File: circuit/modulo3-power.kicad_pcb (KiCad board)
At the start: 2 copper layers, 0 parts

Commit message: fv-1 mostly done; power progressed
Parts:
- added BT1: 25V, myAmp:XT60-M, F.Cu at (107.3, 97.2)
- added C1: 100nF, myAmp:C_1206, F.Cu at (62.9, 67.3)
- added C10: 47μF, myAmp:CPOL_D4_P1.5, F.Cu at (96.5, 59.1)
- added C2: 330n, myAmp:C_5.0MM, F.Cu at (120.7, 85.7)
- added C3: 100nF, myAmp:C_1206, F.Cu at (61.6, 80.0)
- added C4: 20μF, myAmp:CPOL_D6.3_P2.5, F.Cu at (57.1, 80.0)
- added C5: 20μF, myAmp:CPOL_D6.3_P2.5, F.Cu at (66.0, 80.0)
- added C6: 10μF, myAmp:C_1812, F.Cu at (68.6, 64.1)
- added C7: 10μF, myAmp:C_1812, F.Cu at (72.4, 64.1)
- added C8: 100nF, myAmp:C_1206, F.Cu at (96.5, 62.9)
- added C9: 10μF, myAmp:CPOL_D4_P1.5, F.Cu at (101.6, 65.4)
- added D1: 1N4148, myAmp:DO35, F.Cu at (65.4, 64.1)
- added D2: SS18A, myAmp:D_SMA, F.Cu at (57.8, 72.4)
- added D3: power, myAmp:LED_D3.0mm, F.Cu at (92.1, 97.8)
- added F1: 2A, myAmp:MF-LSMF, F.Cu at (106.7, 87.0)
- added J1: HOLE, myAmp:MountingHole, F.Cu at (54.0, 54.0)
- added J2: HOLE, myAmp:MountingHole, F.Cu at (130.0, 54.0)
- added J3: HOLE, myAmp:MountingHole, F.Cu at (54.0, 98.0)
- added J4: HOLE, myAmp:MountingHole, F.Cu at (130.0, 98.0)
- added L1: 27μH, myAmp:COIL_DER0705, F.Cu at (69.2, 72.4)
- added Q1: IRF4905SPBF, myAmp:D2PAK, F.Cu at (120.7, 73.7)
- added R1: 470k, myAmp:R_10MM, F.Cu at (120.7, 88.9)
- added R2: 75K, myAmp:R_0805, F.Cu at (61.0, 62.2)
- added R3: 10K, myAmp:R_0805, F.Cu at (58.4, 62.2)
- added R4: 1M, myAmp:R_10MM, F.Cu at (120.7, 91.4)
- added R5: 4k7, myAmp:R_10MM, F.Cu at (82.5, 97.8)
- added SW1: on/off, myAmp:SW_DPDT, F.Cu at (120.7, 98.0)
- added U1: MCP16331, myAmp:SOT-23-6, F.Cu at (59.7, 67.3)
- added U2: LM1117-5.0, myAmp:TO-252-3, F.Cu at (107.4, 59.7)
- added U3: PWR_CONN, myAmp:PWR_CONN, F.Cu at (121.0, 54.0)
- added U4: AMPCTRL, myAmp:AMPCTRL, F.Cu at (76.0, 54.0)
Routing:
- added copper zone on B.Cu, net GND
- added copper zone on F.Cu, net GND
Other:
- board outline added: 84 x 52 mm

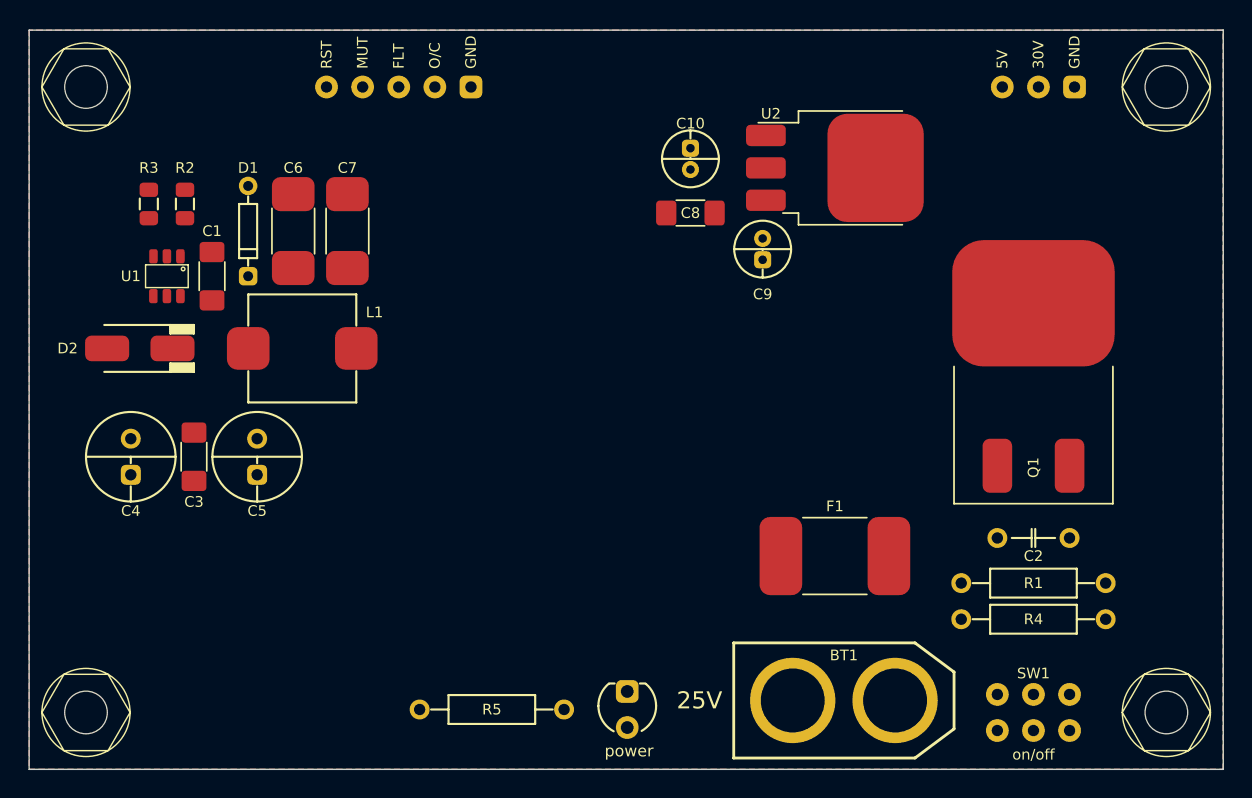
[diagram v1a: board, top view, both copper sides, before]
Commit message: lotsa things :)
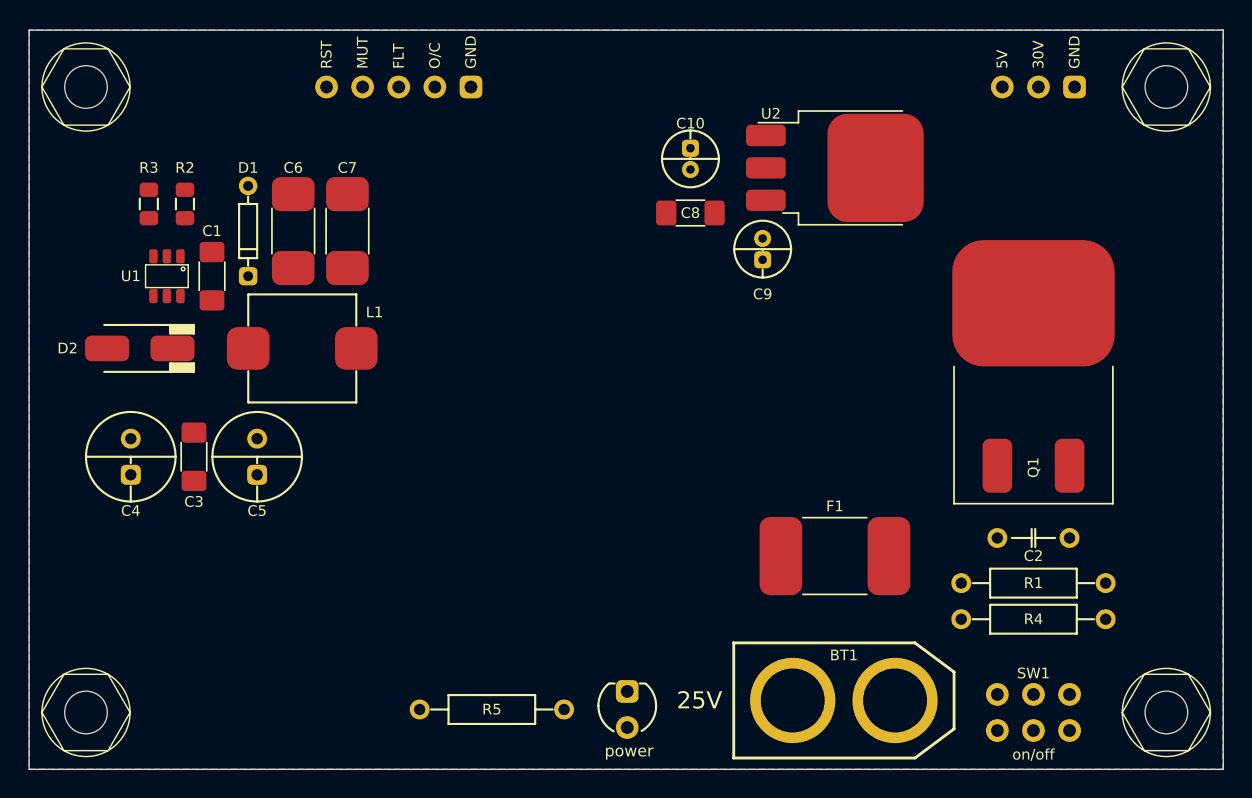
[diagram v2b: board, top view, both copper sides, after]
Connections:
- SW1 pad 5: unconnected-(SW1-Pad5) -> /MUTE
- SW1 pad 6: unconnected-(SW1-Pad6) -> GND
- U4 pad 3: unconnected-(U4-MUTE-Pad3) -> /MUTE
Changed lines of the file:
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@@
   (net 13 "unconnected-(U1-EN-Pad4)")
   (net 14 "unconnected-(U4-RESET-Pad2)")
-  (net 15 "unconnected-(U4-MUTE-Pad3)")
+  (net 15 "/MUTE")
   (net 16 "unconnected-(U4-FAULT-Pad4)")
   (net 17 "unconnected-(U4-OTW_CLIP-Pad5)")
   (net 18 "unconnected-(SW1-Pad3)")
   (net 19 "unconnected-(SW1-Pad4)")
-  (net 20 "unconnected-(SW1-Pad5)")
-  (net 21 "unconnected-(SW1-Pad6)")
   (footprint "myAmp:C_1812" (layer "F.Cu")
     (at 68.58 64.135 90)
@@
         (effects (font (size 0.75 0.75) (thickness 0.15)))
     )
-    (pad "1" thru_hole circle (at -1.27 2.54) (size 1.6 1.6) (drill 0.8) (layers "*.Cu" "*.Mask")
+    (pad "1" thru_hole circle (at -1.27 2.54) (size 1.6 1.6) (drill 0.9) (layers "*.Cu" "*.Mask")
       (net 5 "Net-(Q1-S)") (pintype "passive"))
-    (pad "2" thru_hole circle (at -1.27 0) (size 1.6 1.6) (drill 0.8) (layers "*.Cu" "*.Mask")
+    (pad "2" thru_hole circle (at -1.27 0) (size 1.6 1.6) (drill 0.9) (layers "*.Cu" "*.Mask")
       (net 11 "Net-(F1-Pad2)") (pintype "passive"))
-    (pad "3" thru_hole circle (at -1.27 -2.54) (size 1.6 1.6) (drill 0.8) (layers "*.Cu" "*.Mask")
+    (pad "3" thru_hole circle (at -1.27 -2.54) (size 1.6 1.6) (drill 0.9) (layers "*.Cu" "*.Mask")
       (net 18 "unconnected-(SW1-Pad3)") (pintype "passive+no_connect"))
-    (pad "4" thru_hole circle (at 1.27 2.54) (size 1.6 1.6) (drill 0.8) (layers "*.Cu" "*.Mask")
+    (pad "4" thru_hole circle (at 1.27 2.54) (size 1.6 1.6) (drill 0.9) (layers "*.Cu" "*.Mask")
       (net 19 "unconnected-(SW1-Pad4)") (pintype "passive+no_connect"))
-    (pad "5" thru_hole circle (at 1.27 0) (size 1.6 1.6) (drill 0.8) (layers "*.Cu" "*.Mask")
-      (net 20 "unconnected-(SW1-Pad5)") (pintype "passive"))
-    (pad "6" thru_hole circle (at 1.27 -2.54) (size 1.6 1.6) (drill 0.8) (layers "*.Cu" "*.Mask")
-      (net 21 "unconnected-(SW1-Pad6)") (pintype "passive"))
+    (pad "5" thru_hole circle (at 1.27 0) (size 1.6 1.6) (drill 0.9) (layers "*.Cu" "*.Mask")
+      (net 15 "/MUTE") (pintype "passive"))
+    (pad "6" thru_hole circle (at 1.27 -2.54) (size 1.6 1.6) (drill 0.9) (layers "*.Cu" "*.Mask")
+      (net 1 "GND") (pintype "passive"))
     (model "${KIPRJMOD}/myAmp.pretty/models/PinHeader_2x03_P2.54mm_Horizontal.wrl"
       (offset (xyz -1.27 2.54 0))
@@
     )
   )
-  (footprint "myAmp:AMPCTRL" (layer "F.Cu")
-    (at 76 54)
-    (property "Sheetfile" "modulo3-power.kicad_sch")
-    (property "Sheetname" "")
-    (attr through_hole)
-    (fp_text reference "U4" (at -7.62 0 unlocked) (layer "F.SilkS") hide
-        (effects (font (size 0.75 0.75) (thickness 0.15)))
-    )
-    (fp_text value "AMPCTRL" (at 0 1 unlocked) (layer "F.Fab") hide
-        (effects (font (size 1 1) (thickness 0.15)))
-    )
-    (fp_text user "FLT" (at 0 -1.27 90 unlocked) (layer "F.SilkS")
-        (effects (font (size 0.75 0.75) (thickness 0.15)) (justify left))
-    )
-    (fp_text user "MUT" (at -2.54 -1.27 90 unlocked) (layer "F.SilkS")
-        (effects (font (size 0.75 0.75) (thickness 0.15)) (justify left))
-    )
-    (fp_text user "GND" (at 5.08 -1.27 90 unlocked) (layer "F.SilkS")
-        (effects (font (size 0.75 0.75) (thickness 0.15)) (justify left))
-    )
-    (fp_text user "O/C" (at 2.54 -1.27 90 unlocked) (layer "F.SilkS")
-        (effects (font (size 0.75 0.75) (thickness 0.15)) (justify left))
-    )
-    (fp_text user "RST" (at -5.08 -1.27 90 unlocked) (layer "F.SilkS")
-        (effects (font (size 0.75 0.75) (thickness 0.15)) (justify left))
-    )
-    (pad "1" thru_hole roundrect (at 5.08 0) (size 1.6 1.6) (drill 0.8) (layers "*.Cu" "*.Mask") (roundrect_rratio 0.25)
-      (net 1 "GND") (pinfunction "GND") (pintype "input"))
-    (pad "2" thru_hole circle (at -5.08 0) (size 1.6 1.6) (drill 0.8) (layers "*.Cu" "*.Mask")
-      (net 14 "unconnected-(U4-RESET-Pad2)") (pinfunction "RESET") (pintype "input"))
-    (pad "3" thru_hole circle (at -2.54 0) (size 1.6 1.6) (drill 0.8) (layers "*.Cu" "*.Mask")
-      (net 15 "unconnected-(U4-MUTE-Pad3)") (pinfunction "MUTE") (pintype "input"))
-    (pad "4" thru_hole circle (at 0 0) (size 1.6 1.6) (drill 0.8) (layers "*.Cu" "*.Mask")
-      (net 16 "unconnected-(U4-FAULT-Pad4)") (pinfunction "FAULT") (pintype "output+no_connect"))
-    (pad "5" thru_hole circle (at 2.54 0) (size 1.6 1.6) (drill 0.8) (layers "*.Cu" "*.Mask")
-      (net 17 "unconnected-(U4-OTW_CLIP-Pad5)") (pinfunction "OTW_CLIP") (pintype "output+no_connect"))
-    (model "${KIPRJMOD}/myAmp.pretty/models/PinHeader_1x05_P2.54mm_Vertical.wrl"
-      (offset (xyz 5.08 0 0))
-      (scale (xyz 1 1 1))
-      (rotate (xyz 0 0 90))
-    )
-  )
   (footprint "myAmp:MountingHole" (layer "F.Cu")
     (at 54 54)
@@
       (scale (xyz 1 1 1))
       (rotate (xyz 0 0 0))
+    )
+  )
+  (footprint "myAmp:AMPCTRL" (layer "F.Cu")
+    (at 76 54)
+    (property "Sheetfile" "modulo3-power.kicad_sch")
+    (property "Sheetname" "")
+    (attr through_hole)
+    (fp_text reference "U4" (at -7.62 0 unlocked) (layer "F.SilkS") hide
+        (effects (font (size 0.75 0.75) (thickness 0.15)))
+    )
+    (fp_text value "AMPCTRL" (at 0 1 unlocked) (layer "F.Fab") hide
+        (effects (font (size 1 1) (thickness 0.15)))
+    )
+    (fp_text user "O/C" (at 2.54 -1.27 90 unlocked) (layer "F.SilkS")
+        (effects (font (size 0.75 0.75) (thickness 0.15)) (justify left))
+    )
+    (fp_text user "RST" (at -5.08 -1.27 90 unlocked) (layer "F.SilkS")
+        (effects (font (size 0.75 0.75) (thickness 0.15)) (justify left))
+    )
+    (fp_text user "FLT" (at 0 -1.27 90 unlocked) (layer "F.SilkS")
+        (effects (font (size 0.75 0.75) (thickness 0.15)) (justify left))
+    )
+    (fp_text user "GND" (at 5.08 -1.27 90 unlocked) (layer "F.SilkS")
+        (effects (font (size 0.75 0.75) (thickness 0.15)) (justify left))
+    )
+    (fp_text user "MUT" (at -2.54 -1.27 90 unlocked) (layer "F.SilkS")
+        (effects (font (size 0.75 0.75) (thickness 0.15)) (justify left))
+    )
+    (pad "1" thru_hole roundrect (at 5.08 0) (size 1.6 1.6) (drill 0.9) (layers "*.Cu" "*.Mask") (roundrect_rratio 0.25)
+      (net 1 "GND") (pinfunction "GND") (pintype "input"))
+    (pad "2" thru_hole circle (at -5.08 0) (size 1.6 1.6) (drill 0.9) (layers "*.Cu" "*.Mask")
+      (net 14 "unconnected-(U4-RESET-Pad2)") (pinfunction "RESET") (pintype "input+no_connect"))
+    (pad "3" thru_hole circle (at -2.54 0) (size 1.6 1.6) (drill 0.9) (layers "*.Cu" "*.Mask")
+      (net 15 "/MUTE") (pinfunction "MUTE") (pintype "input"))
+    (pad "4" thru_hole circle (at 0 0) (size 1.6 1.6) (drill 0.9) (layers "*.Cu" "*.Mask")
+      (net 16 "unconnected-(U4-FAULT-Pad4)") (pinfunction "FAULT") (pintype "output+no_connect"))
+    (pad "5" thru_hole circle (at 2.54 0) (size 1.6 1.6) (drill 0.9) (layers "*.Cu" "*.Mask")
+      (net 17 "unconnected-(U4-OTW_CLIP-Pad5)") (pinfunction "OTW_CLIP") (pintype "output+no_connect"))
+    (model "${KIPRJMOD}/myAmp.pretty/models/PinHeader_1x05_P2.54mm_Vertical.wrl"
+      (offset (xyz 5.08 0 0))
+      (scale (xyz 1 1 1))
+      (rotate (xyz 0 0 90))
     )
   )
@@
         (effects (font (size 0.75 0.75) (thickness 0.15)) (justify left))
     )
-    (pad "1" thru_hole roundrect (at 2.54 0 180) (size 1.6 1.6) (drill 0.8) (layers "*.Cu" "*.Mask") (roundrect_rratio 0.25)
+    (pad "1" thru_hole roundrect (at 2.54 0 180) (size 1.6 1.6) (drill 0.9) (layers "*.Cu" "*.Mask") (roundrect_rratio 0.25)
       (net 1 "GND") (pinfunction "GND") (pintype "passive"))
-    (pad "2" thru_hole circle (at 0 0 180) (size 1.6 1.6) (drill 0.8) (layers "*.Cu" "*.Mask")
+    (pad "2" thru_hole circle (at 0 0 180) (size 1.6 1.6) (drill 0.9) (layers "*.Cu" "*.Mask")
       (net 7 "+BATT") (pinfunction "30V") (pintype "passive"))
-    (pad "3" thru_hole circle (at -2.54 0 180) (size 1.6 1.6) (drill 0.8) (layers "*.Cu" "*.Mask")
+    (pad "3" thru_hole circle (at -2.54 0 180) (size 1.6 1.6) (drill 0.9) (layers "*.Cu" "*.Mask")
       (net 9 "+5V") (pinfunction "5V") (pintype "passive"))
     (model "${KIPRJMOD}/myAmp.pretty/models/PinHeader_1x03_P2.54mm_Vertical.step"
@@
     (stroke (width 0.1) (type default)) (layer "Edge.Cuts"))
   (zone (net 1) (net_name "GND") (layers "F&B.Cu") (hatch edge 0.5)
-    (connect_pads (clearance 0.5))
-    (min_thickness 0.25) (filled_areas_thickness no)
-    (fill yes (thermal_gap 0.5) (thermal_bridge_width 0.5))
+    (connect_pads (clearance 0.254))
+    (min_thickness 0.254) (filled_areas_thickness no)
+    (fill yes (thermal_gap 0.254) (thermal_bridge_width 0.254))
     (polygon
       (pts
